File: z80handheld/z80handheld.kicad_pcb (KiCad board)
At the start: 2 copper layers, 107.9 x 151.1 mm, 139 parts, among them IC1 DS12885+, J1 Power, J2 Esp32 C3 Supermini Right, J3 SPI Screen, J4 Esp32 C3 Supermini Left, J5 Conn_01x40, SW1 SW_Push_45deg, SW10 SW_Push_45deg, SW11 SW_Push_45deg, SW12 SW_Push_45deg, SW13 SW_Push_45deg, SW14 SW_Push_45deg, SW15 SW_Push_45deg, SW16 SW_Push_45deg, SW17 SW_Push_45deg, SW18 SW_Push_45deg, SW19 SW_Push_45deg, SW2 SW_Push_45deg, SW20 SW_Push_45deg, SW21 SW_Push_45deg, SW22 SW_Push_45deg, SW23 SW_Push_45deg, SW24 SW_Push_45deg, SW25 SW_Push_45deg, SW26 SW_Push_45deg, SW27 SW_Push_45deg, SW28 SW_Push_45deg, SW29 SW_Push_45deg, SW3 SW_Push_45deg, SW30 SW_Push_45deg, SW31 SW_Push_45deg, SW32 SW_Push_45deg, SW33 SW_Push_45deg, SW34 SW_Push_45deg, SW35 SW_Push_45deg, SW36 SW_Push_45deg, SW37 SW_Push_45deg, SW38 SW_Push_45deg, SW39 SW_Push_45deg, SW4 SW_Push_45deg, SW40 SW_Push_45deg, SW41 SW_Push_45deg, SW42 SW_Push_45deg, SW43 SW_Push_45deg, SW44 SW_Push_45deg, SW45 SW_Push_45deg, SW46 SW_Push_45deg, SW47 SW_Push_45deg, SW48 SW_Push_45deg, SW49 SW_Push_45deg, SW5 SW_Push_45deg, SW50 SW_Push_45deg, SW51 SW_Push_45deg, SW52 SW_Push_45deg, SW53 SW_Push_45deg, SW54 SW_Push_45deg, SW55 SW_Push_45deg, SW56 SW_Push_45deg, SW57 SW_Push_45deg, SW58 SW_Push_45deg, SW59 SW_Push_45deg, SW6 SW_Push_45deg, SW60 SW_Push_45deg, SW61 SW_Push_45deg, SW62 SW_Push_45deg, SW63 SW_Push_45deg, SW64 SW_Push_45deg, SW65 SW_Push, SW7 SW_Push_45deg, SW8 SW_Push_45deg, SW9 SW_Push_45deg, U1 74HC04, U10 Z84C00xxP, U11 74LS573 IO1, U12 HDSP-7501, U13 74LS573, U14 HDSP-7501, U15 74LS573, U16 16550 IO2, U17 16550 IO3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

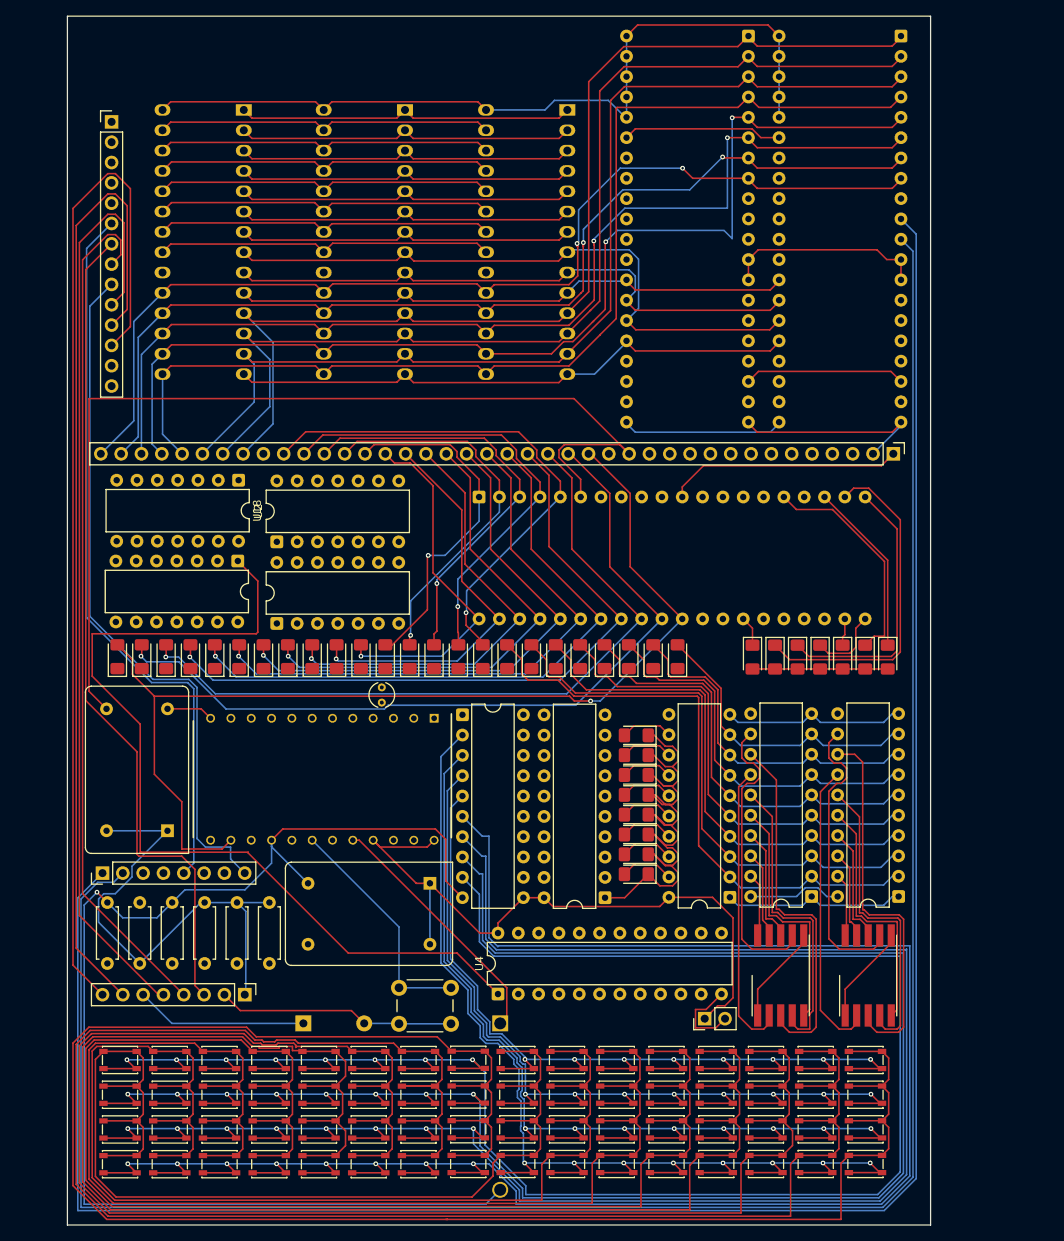
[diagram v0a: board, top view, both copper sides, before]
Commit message: Add files via upload
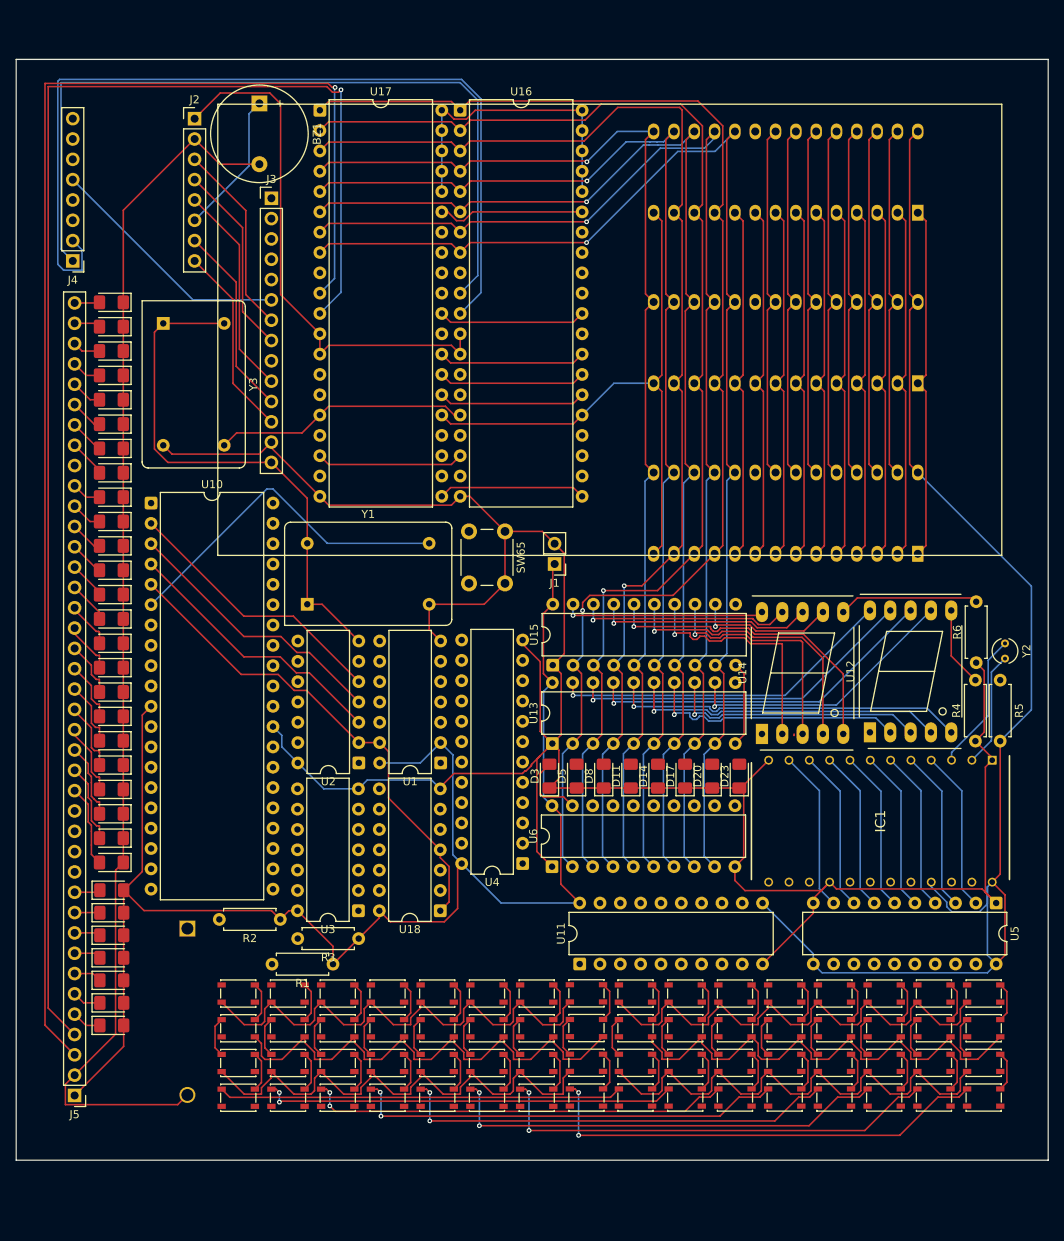
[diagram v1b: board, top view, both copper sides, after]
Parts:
- BZ1, U10, U16, U17: moved to F.Cu
- U12, U14: footprint Display_7Segment:KCSC02-106 -> Display_7Segment:7SegmentLED_LTS6760_LTS6780
- moved J5 130.0 mm to (204.7, 202.2), turned to 180 degrees
- moved BZ1 115.1 mm to (227.8, 78.2), turned to -90 degrees
- moved R6 112.7 mm to (317.4, 148.1), turned to 90 degrees
- moved R5 111.1 mm to (320.4, 150.3)
- moved J2 109.7 mm to (219.7, 80.1), turned to 0 degrees
- moved R4 102.4 mm to (317.3, 157.9), turned to 90 degrees
- moved D6 101.3 mm to (209.3, 176.6), turned to 0 degrees
- moved D9 99.5 mm to (209.3, 179.4), turned to 0 degrees
- moved D12 97.8 mm to (209.3, 182.2), turned to 0 degrees
- moved D15 96.2 mm to (209.3, 185.0), turned to 0 degrees
- moved D18 94.8 mm to (209.3, 187.8), turned to 0 degrees
- moved D21 93.5 mm to (209.3, 190.6), turned to 0 degrees
- moved D24 92.4 mm to (209.3, 193.4), turned to 0 degrees
- moved U9 85.2 mm to (310.1, 91.9), turned to 90 degrees
- moved U7 84.8 mm to (310.1, 134.5), turned to 90 degrees
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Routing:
- net Net-(U11-D4): track 247.4 -> 0.00 mm, vias 8 -> 0
- net 5V: track 331.9 -> 542.2 mm
- net TX2: track 0.00 -> 185.9 mm, vias 0 -> 1
- net RX2: track 0.00 -> 185.9 mm, vias 0 -> 1
- net Net-(U11-D7): track 246.4 -> 66.3 mm, vias 8 -> 0
- net Net-(U11-D6): track 246.3 -> 66.3 mm, vias 8 -> 0
- net Net-(U11-D5): track 246.4 -> 66.6 mm, vias 8 -> 0
- net TX1: track 270.7 -> 100.9 mm
- net RX1: track 268.5 -> 112.3 mm
- net Net-(U11-D0): track 149.6 -> 0.00 mm, vias 8 -> 0
- net Net-(U5-Q0): track 236.9 -> 87.7 mm, vias 0 -> 2
- net Net-(U5-Q1): track 226.7 -> 86.9 mm, vias 0 -> 2
- net /A0: track 201.7 -> 73.0 mm, vias 1 -> 0
- net GND: track 419.8 -> 542.9 mm, vias 1 -> 0
- net Net-(U5-Q2): track 208.9 -> 86.0 mm, vias 0 -> 2
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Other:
- board size 107.9 x 151.1 mm -> 129 x 137.6 mm
- board text removed: "!BANK_0 !BANK_1 SIGNALS"
